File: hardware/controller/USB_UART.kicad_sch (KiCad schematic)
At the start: 1 part, among them IC1 CY7C65213-32LTXI

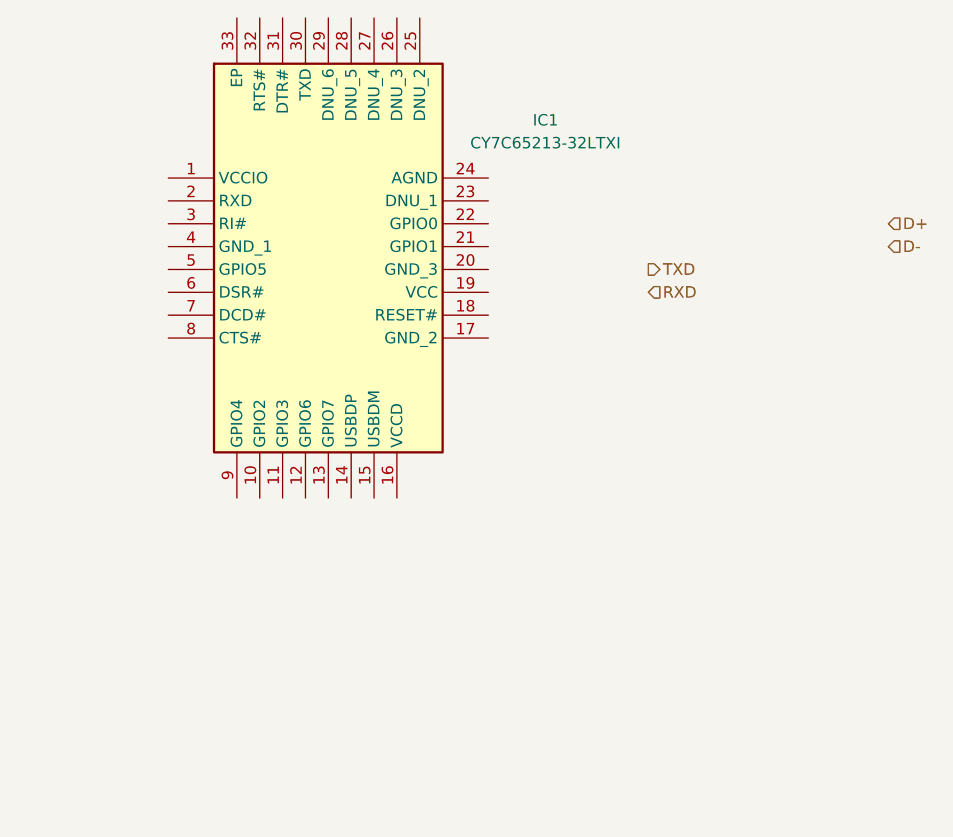
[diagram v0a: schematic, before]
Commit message: a
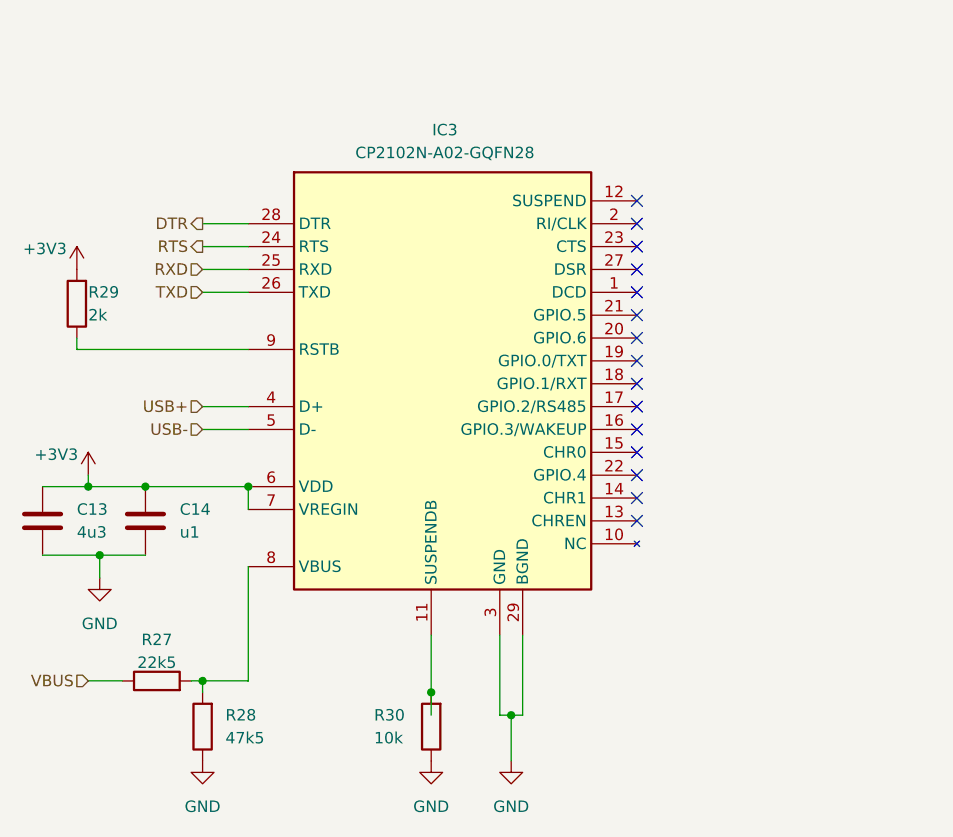
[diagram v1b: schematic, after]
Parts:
- removed IC1: CY7C65213-32LTXI, QFN50P500X500X100-33N-D, symbol SamacSys_Parts:CY7C65213-32LTXI
- added C13: 4u3, symbol Device:C
- added C14: u1, symbol Device:C
- added IC3: CP2102N-A02-GQFN28, QFN50P500X500X80-29N-D, symbol SamacSys_Parts:CP2102N-A02-GQFN28
- added R27: 22k5, symbol Device:R
- added R28: 47k5, symbol Device:R
- added R29: 2k, symbol Device:R
- added R30: 10k, symbol Device:R
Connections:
- net RXD: now also IC3.25 (RXD)
- net TXD: now also IC3.26 (TXD)
- new net: IC3.11 (SUSPENDB), R30.2
- new net: IC3.8 (VBUS), R27.2, R28.2
- new net: IC3.9 (RSTB), R29.1
- new net +3V3: C13.1, C14.1, IC3.6 (VDD), IC3.7 (VREGIN), R29.2
- new net DTR: IC3.28 (DTR)
- new net GND: C13.2, C14.2, IC3.29 (BGND), IC3.3 (GND), R28.1, R30.1
- new net RTS: IC3.24 (RTS)
- new net USB+: IC3.4 (D+)
- new net USB-: IC3.5 (D-)
- new net VBUS: R27.1
- no-connect marks 0 -> 15
